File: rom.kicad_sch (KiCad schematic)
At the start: 7 parts, among them U10 28C256, U6 74HC32, U7 74HC14, U8 74HC05, U9 28C256

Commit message: done the pcb layout + added the 1M ram bank project
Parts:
- C1: footprint Capacitor_THT:C_Disc_P2.54mm -> Capacitor_THT:C_Disc_D3.0mm_W1.6mm_P2.54mm
- U10, U9: footprint Package_DIP:DIP-28_W15.24mm_Socket -> Package_DIP:DIP-28_W15.24mm
- U6, U7, U8: footprint Package_DIP:DIP-14_W7.62mm_Socket -> Package_DIP:DIP-14_W7.62mm
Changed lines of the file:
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@@
 			)
 		)
-		(property "Footprint" "Package_DIP:DIP-14_W7.62mm_Socket"
+		(property "Footprint" "Package_DIP:DIP-14_W7.62mm"
 			(at 76.2 142.24 0)
 			(effects
@@
 			)
 		)
-		(property "Footprint" "Package_DIP:DIP-28_W15.24mm_Socket"
+		(property "Footprint" "Package_DIP:DIP-28_W15.24mm"
 			(at 152.4 101.6 0)
 			(effects
@@
 			)
 		)
-		(property "Footprint" "Package_DIP:DIP-14_W7.62mm_Socket"
+		(property "Footprint" "Package_DIP:DIP-14_W7.62mm"
 			(at 71.12 76.2 0)
 			(effects
@@
 			)
 		)
-		(property "Footprint" "Package_DIP:DIP-28_W15.24mm_Socket"
+		(property "Footprint" "Package_DIP:DIP-28_W15.24mm"
 			(at 215.9 101.6 0)
 			(effects
@@
 			)
 		)
-		(property "Footprint" "Capacitor_THT:C_Disc_P2.54mm"
+		(property "Footprint" "Capacitor_THT:C_Disc_D3.0mm_W1.6mm_P2.54mm"
 			(at 86.36 75.2348 0)
 			(effects
@@
 			)
 		)
-		(property "Footprint" "Package_DIP:DIP-14_W7.62mm_Socket"
+		(property "Footprint" "Package_DIP:DIP-14_W7.62mm"
 			(at 76.2 149.86 0)
 			(effects
@@
 			)
 		)
-		(property "Footprint" "Package_DIP:DIP-14_W7.62mm_Socket"
+		(property "Footprint" "Package_DIP:DIP-14_W7.62mm"
 			(at 93.98 76.2 0)
 			(effects

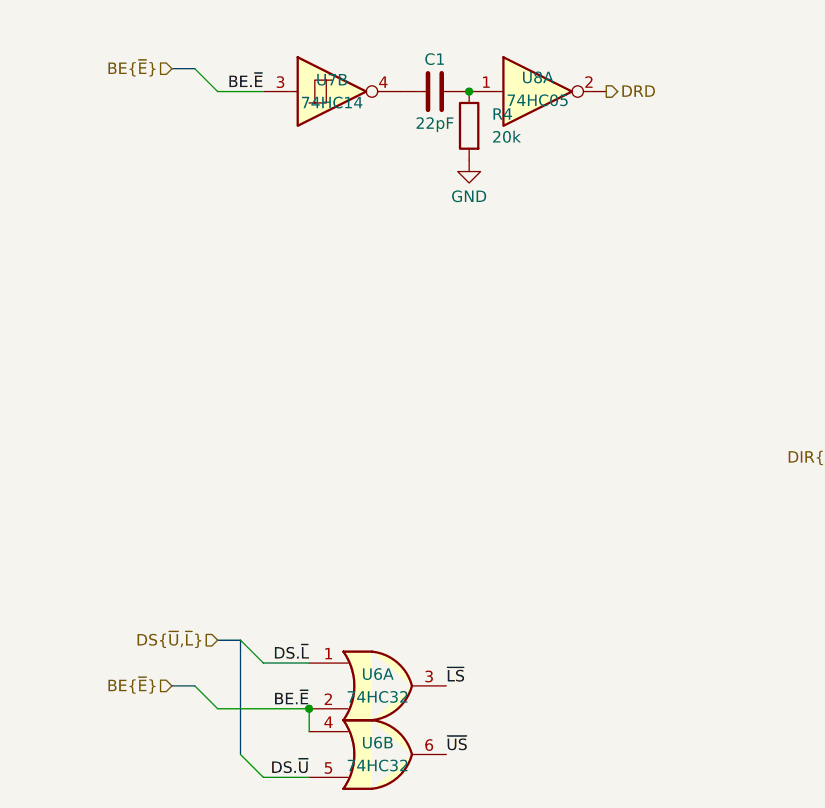
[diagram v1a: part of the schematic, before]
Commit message: [scheme] no major changes
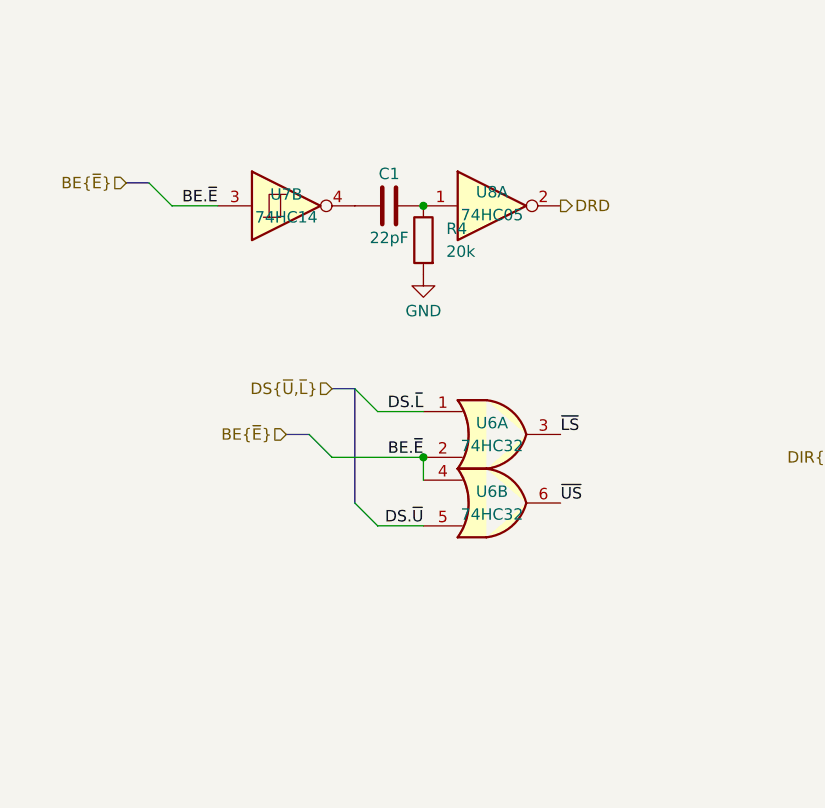
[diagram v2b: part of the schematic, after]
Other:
- moved on the sheet: C1, R4, U6A, U6B, U7B, U8A
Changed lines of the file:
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@@
 	(paper "A4")
 	(junction
-		(at 68.58 144.78)
+		(at 81.28 116.84)
 		(diameter 0)
 		(color 0 0 0 0)
 	)
 	(junction
-		(at 86.36 76.2)
+		(at 81.28 88.9)
 		(diameter 0)
 		(color 0 0 0 0)
@@
 	)
 	(bus_entry
-		(at 60.96 149.86)
+		(at 73.66 121.92)
 		(size 2.54 2.54)
 		(stroke
@@
 	)
 	(bus_entry
-		(at 55.88 142.24)
+		(at 68.58 114.3)
 		(size 2.54 2.54)
 		(stroke
@@
 	)
 	(bus_entry
-		(at 55.88 73.66)
+		(at 50.8 86.36)
 		(size 2.54 2.54)
 		(stroke
@@
 	)
 	(bus_entry
-		(at 60.96 137.16)
+		(at 73.66 109.22)
 		(size 2.54 2.54)
 		(stroke
@@
 	(bus
 		(pts
-			(xy 53.34 142.24) (xy 55.88 142.24)
+			(xy 66.04 114.3) (xy 68.58 114.3)
 		)
 		(stroke
@@
 	(wire
 		(pts
-			(xy 58.42 144.78) (xy 68.58 144.78)
+			(xy 71.12 116.84) (xy 81.28 116.84)
 		)
 		(stroke
@@
 	(bus
 		(pts
-			(xy 53.34 73.66) (xy 55.88 73.66)
+			(xy 48.26 86.36) (xy 50.8 86.36)
 		)
 		(stroke
@@
 	(wire
 		(pts
-			(xy 68.58 144.78) (xy 68.58 147.32)
+			(xy 81.28 116.84) (xy 81.28 119.38)
 		)
 		(stroke
@@
 	(wire
 		(pts
-			(xy 58.42 76.2) (xy 63.5 76.2)
+			(xy 53.34 88.9) (xy 58.42 88.9)
 		)
 		(stroke
@@
 	(wire
 		(pts
-			(xy 63.5 139.7) (xy 68.58 139.7)
+			(xy 76.2 111.76) (xy 81.28 111.76)
 		)
 		(stroke
@@
 	(wire
 		(pts
-			(xy 63.5 152.4) (xy 68.58 152.4)
+			(xy 76.2 124.46) (xy 81.28 124.46)
 		)
 		(stroke
@@
 	(bus
 		(pts
-			(xy 60.96 137.16) (xy 60.96 149.86)
+			(xy 73.66 109.22) (xy 73.66 121.92)
 		)
 		(stroke
@@
 	(bus
 		(pts
-			(xy 58.42 137.16) (xy 60.96 137.16)
+			(xy 71.12 109.22) (xy 73.66 109.22)
 		)
 		(stroke
@@
 	)
 	(label "~{US}"
-		(at 83.82 149.86 0)
+		(at 96.52 121.92 0)
 		(effects
 			(font
@@
 	)
 	(label "BE.~{E}"
-		(at 63.5 76.2 180)
+		(at 58.42 88.9 180)
 		(effects
 			(font
@@
 	)
 	(label "~{LS}"
-		(at 83.82 142.24 0)
+		(at 96.52 114.3 0)
 		(effects
 			(font
@@
 	)
 	(label "BE.~{E}"
-		(at 68.58 144.78 180)
+		(at 81.28 116.84 180)
 		(effects
 			(font
@@
 	)
 	(label "DS.~{L}"
-		(at 68.58 139.7 180)
+		(at 81.28 111.76 180)
 		(effects
 			(font
@@
 	)
 	(label "DS.~{U}"
-		(at 68.58 152.4 180)
+		(at 81.28 124.46 180)
 		(effects
 			(font
@@
 	(hierarchical_label "BE{~{E}}"
 		(shape input)
-		(at 53.34 142.24 180)
+		(at 66.04 114.3 180)
 		(effects
 			(font
@@
 	(hierarchical_label "BE{~{E}}"
 		(shape input)
-		(at 53.34 73.66 180)
+		(at 48.26 86.36 180)
 		(effects
 			(font
@@
 	(hierarchical_label "DS{~{U},~{L}}"
 		(shape input)
-		(at 58.42 137.16 180)
+		(at 71.12 109.22 180)
 		(effects
 			(font
@@
 	(hierarchical_label "DRD"
 		(shape output)
-		(at 101.6 76.2 0)
+		(at 96.52 88.9 0)
 		(effects
 			(font
@@
 	(symbol
 		(lib_id "74xx:74LS32")
-		(at 76.2 142.24 0)
+		(at 88.9 114.3 0)
 		(unit 1)
 		(exclude_from_sim no)
@@
 		(dnp no)
 		(property "Reference" "U6"
-			(at 76.2 140.97 0)
+			(at 88.9 113.03 0)
 			(effects
 				(font
@@
 		)
 		(property "Value" "74HC32"
-			(at 76.2 143.51 0)
+			(at 88.9 115.57 0)
 			(effects
 				(font
@@
 		)
 		(property "Footprint" "Package_DIP:DIP-14_W7.62mm"
-			(at 76.2 142.24 0)
+			(at 88.9 114.3 0)
 			(effects
 				(font
@@
 		)
 		(property "Datasheet" "http://www.ti.com/lit/gpn/sn74LS32"
-			(at 76.2 142.24 0)
+			(at 88.9 114.3 0)
 			(effects
 				(font
@@
 		)
 		(property "Description" "Quad 2-input OR"
-			(at 76.2 142.24 0)
+			(at 88.9 114.3 0)
 			(effects
 				(font
@@
 	(symbol
 		(lib_id "Device:R")
-		(at 86.36 80.01 0)
+		(at 81.28 92.71 0)
 		(mirror y)
 		(unit 1)
@@
 		(dnp no)
 		(property "Reference" "R4"
-			(at 88.9 78.7399 0)
+			(at 83.82 91.4399 0)
 			(effects
 				(font
@@
 		)
 		(property "Value" "20k"
-			(at 88.9 81.2799 0)
+			(at 83.82 93.9799 0)
 			(effects
 				(font
@@
 		)
 		(property "Footprint" "Resistor_THT:R_Axial_DIN0207_L6.3mm_D2.5mm_P2.54mm_Vertical"
-			(at 88.138 80.01 90)
+			(at 83.058 92.71 90)
 			(effects
 				(font
@@
 		)
 		(property "Datasheet" "~"
-			(at 86.36 80.01 0)
+			(at 81.28 92.71 0)
 			(effects
 				(font
@@
 		)
 		(property "Description" "Resistor"
-			(at 86.36 80.01 0)
+			(at 81.28 92.71 0)
 			(effects
 				(font
@@
 	(symbol
 		(lib_id "74xx:74HC14")
-		(at 71.12 76.2 0)
+		(at 66.04 88.9 0)
 		(unit 2)
 		(exclude_from_sim no)
@@
 		(dnp no)
 		(property "Reference" "U7"
-			(at 71.12 74.93 0)
+			(at 66.04 87.63 0)
 			(effects
 				(font
@@
 		)
 		(property "Value" "74HC14"
-			(at 71.12 77.47 0)
+			(at 66.04 90.17 0)
 			(effects
 				(font
@@
 		)
 		(property "Footprint" "Package_DIP:DIP-14_W7.62mm"
-			(at 71.12 76.2 0)
+			(at 66.04 88.9 0)
 			(effects
 				(font
@@
 		)
 		(property "Datasheet" "http://www.ti.com/lit/gpn/sn74HC14"
-			(at 71.12 76.2 0)
+			(at 66.04 88.9 0)
 			(effects
 				(font
@@
 		)
 		(property "Description" "Hex inverter schmitt trigger"
-			(at 71.12 76.2 0)
+			(at 66.04 88.9 0)
 			(effects
 				(font
@@
 	(symbol
 		(lib_id "Device:C")
-		(at 82.55 76.2 90)
+		(at 77.47 88.9 90)
 		(unit 1)
 		(exclude_from_sim no)
@@
 		(dnp no)
 		(property "Reference" "C1"
-			(at 82.55 72.644 90)
+			(at 77.47 85.344 90)
 			(effects
 				(font
@@
 		)
 		(property "Value" "22pF"
-			(at 82.55 79.756 90)
+			(at 77.47 92.456 90)
 			(effects
 				(font
@@
 		)
 		(property "Footprint" "Capacitor_THT:C_Disc_D3.0mm_W1.6mm_P2.54mm"
-			(at 86.36 75.2348 0)
+			(at 81.28 87.9348 0)
 			(effects
 				(font
@@
 		)
 		(property "Datasheet" "~"
-			(at 82.55 76.2 0)
+			(at 77.47 88.9 0)
 			(effects
 				(font
@@
 		)
 		(property "Description" "Unpolarized capacitor"
-			(at 82.55 76.2 0)
+			(at 77.47 88.9 0)
 			(effects
 				(font
@@
 	(symbol
 		(lib_id "power:GND")
-		(at 86.36 83.82 0)
+		(at 81.28 96.52 0)
 		(mirror y)
 		(unit 1)
@@
 		(dnp no)
 		(property "Reference" "#PWR027"
-			(at 86.36 90.17 0)
+			(at 81.28 102.87 0)
 			(effects
 				(font
@@
 		)
 		(property "Value" "GND"
-			(at 86.36 87.884 0)
+			(at 81.28 100.584 0)
 			(effects
 				(font
@@
 		)
 		(property "Footprint" ""
-			(at 86.36 83.82 0)
+			(at 81.28 96.52 0)
 			(effects
 				(font
@@
 		)
 		(property "Datasheet" ""
-			(at 86.36 83.82 0)
+			(at 81.28 96.52 0)
 			(effects
 				(font
@@
 		)
 		(property "Description" "Power symbol creates a global label with name \"GND\" , ground"
-			(at 86.36 83.82 0)
+			(at 81.28 96.52 0)
 			(effects
 				(font
@@
 	(symbol
 		(lib_id "74xx:74LS32")
-		(at 76.2 149.86 0)
+		(at 88.9 121.92 0)
 		(unit 2)
 		(exclude_from_sim no)
@@
 		(dnp no)
 		(property "Reference" "U6"
-			(at 76.2 148.59 0)
+			(at 88.9 120.65 0)
 			(effects
 				(font
@@
 		)
 		(property "Value" "74HC32"
-			(at 76.2 151.13 0)
+			(at 88.9 123.19 0)
 			(effects
 				(font
@@
 		)
 		(property "Footprint" "Package_DIP:DIP-14_W7.62mm"
-			(at 76.2 149.86 0)
+			(at 88.9 121.92 0)
 			(effects
 				(font
@@
 		)
 		(property "Datasheet" "http://www.ti.com/lit/gpn/sn74LS32"
-			(at 76.2 149.86 0)
+			(at 88.9 121.92 0)
 			(effects
 				(font
@@
 		)
 		(property "Description" "Quad 2-input OR"
-			(at 76.2 149.86 0)
+			(at 88.9 121.92 0)
 			(effects
 				(font
@@
 	(symbol
 		(lib_id "74xx:74LS05")
-		(at 93.98 76.2 0)
+		(at 88.9 88.9 0)
 		(unit 1)
 		(exclude_from_sim no)
@@
 		(dnp no)
 		(property "Reference" "U8"
-			(at 93.98 74.676 0)
+			(at 88.9 87.376 0)
 			(effects
 				(font
@@
 		)
 		(property "Value" "74HC05"
-			(at 93.98 77.216 0)
+			(at 88.9 89.916 0)
 			(effects
 				(font
@@
 		)
 		(property "Footprint" "Package_DIP:DIP-14_W7.62mm"
-			(at 93.98 76.2 0)
+			(at 88.9 88.9 0)
 			(effects
 				(font
@@
 		)
 		(property "Datasheet" "http://www.ti.com/lit/gpn/sn74LS05"
-			(at 93.98 76.2 0)
+			(at 88.9 88.9 0)
 			(effects
 				(font
@@
 		)
 		(property "Description" "Inverter Open Collect"
-			(at 93.98 76.2 0)
-			(effects
-				(font
+			(at 88.9 88.9 0)
+			(effects
+				(font
